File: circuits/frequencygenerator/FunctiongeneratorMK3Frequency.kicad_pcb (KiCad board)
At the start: 2 copper layers, 101.6 x 79 mm, 43 parts, among them J1 FreqRange, J10 50 Ohm OUT, J11 OUT Gain 10k, J12 WaveA2, J13 MO, J2 WaveA1, J3 12V-GND-5V, J4 FreqCounterD5, J5 TTL OUT, J6 SIN-TRI-SQU-PWM, J7 PulseWidth 100k, J8 FreqCoarse 1M, J9 FreqFine 10k, U1 LTV-847, U2 XR2206CP-F, U3 74HC14, U4 NE5532, U5 NE5532

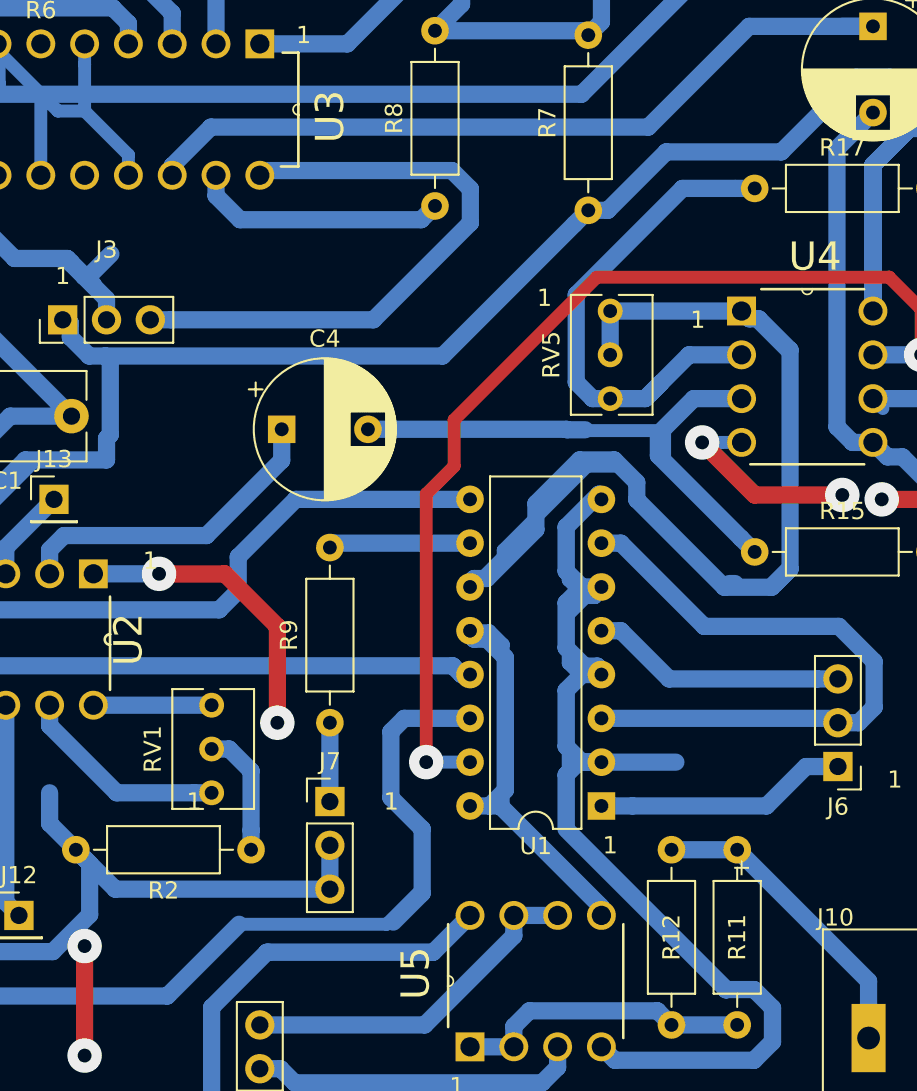
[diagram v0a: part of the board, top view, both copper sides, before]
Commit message: circuit kicad updates
updated circuits to last kicad version

Signed-off-by: Rene Lange <rine@rine.de>
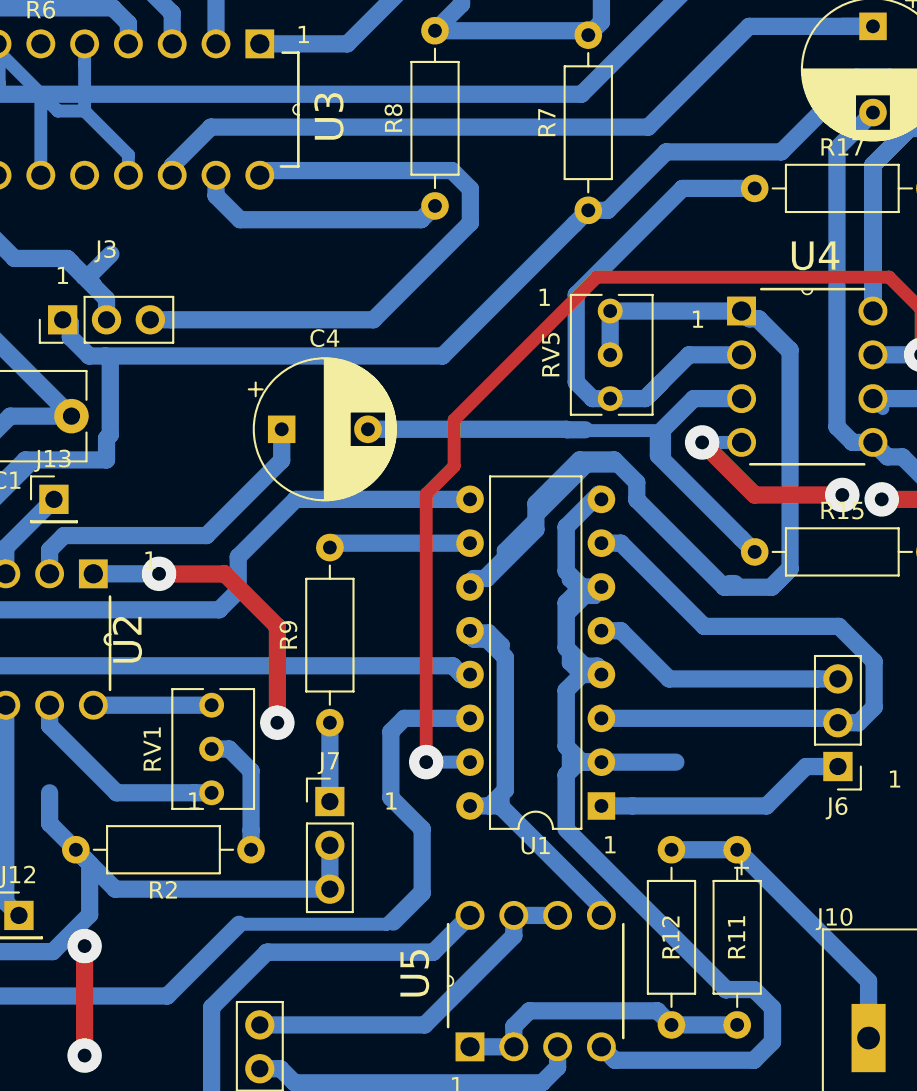
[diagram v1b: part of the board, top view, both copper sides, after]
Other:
- net class Default removed
